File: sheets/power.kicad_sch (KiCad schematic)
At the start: 73 parts, among them SW2 FCC-0001SW, T1 COIL, U11 74LS05, U12 74LS06, U28 PC4741, U29 PC4741, U33 74AS04, U37 LM2576T-5, U38 74HC32, U8 74HC04, U80 74HC04

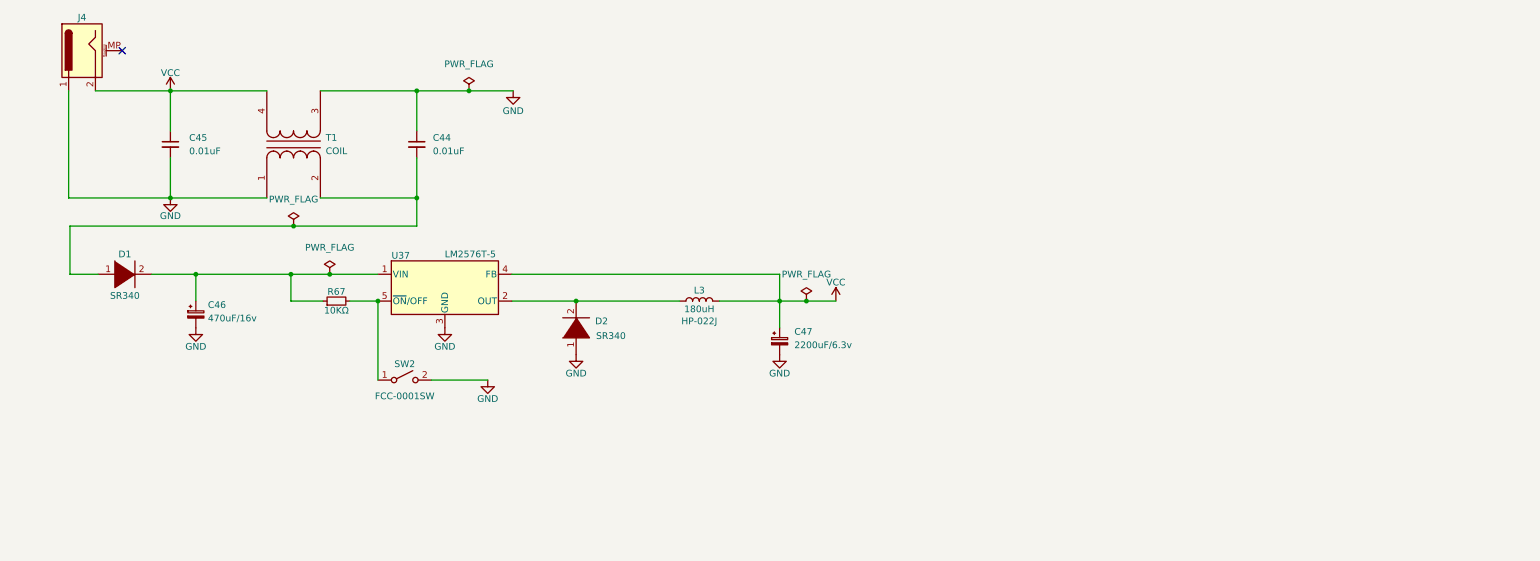
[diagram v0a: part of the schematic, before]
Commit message: Power Circuit Update 1
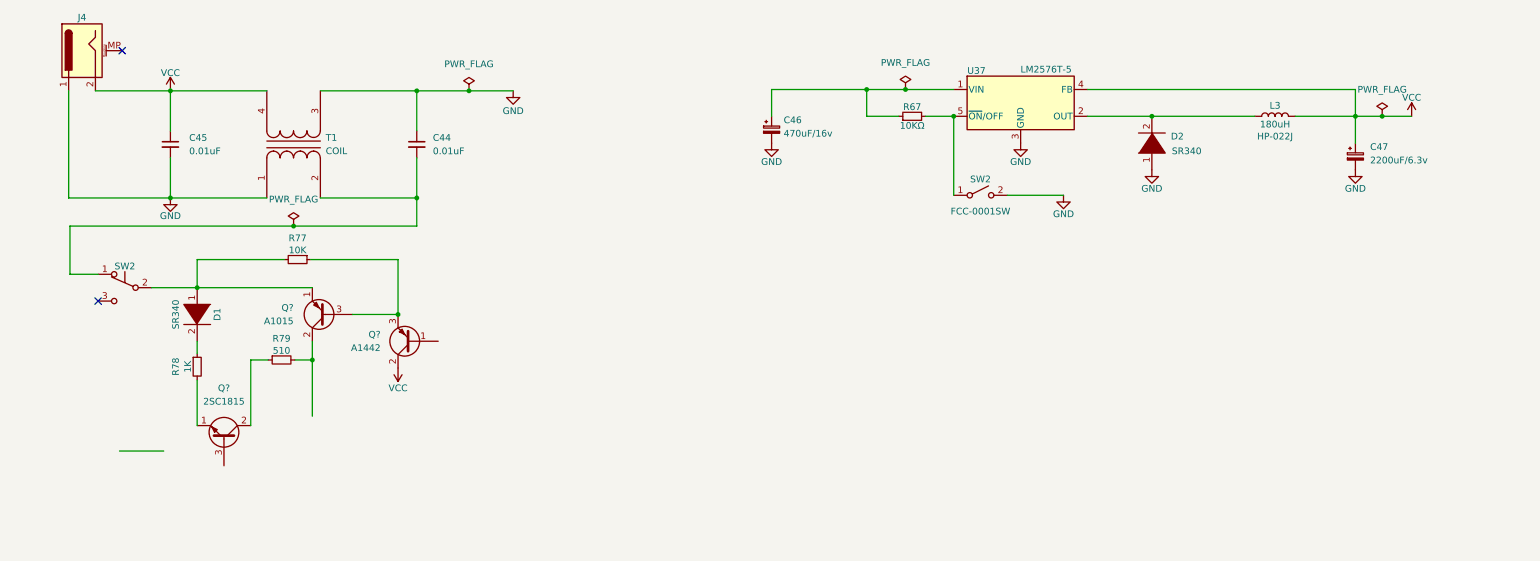
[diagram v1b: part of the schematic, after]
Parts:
- added Q?: A1442, symbol Device:Q_PNP_BCE
- added Q?: A1015, Package_TO_SOT_THT:TO-92_Inline, symbol Transistor_BJT:2SA1015
- added Q?: 2SC1815, Package_TO_SOT_THT:TO-92_Inline, symbol Transistor_BJT:2SC1815
- added R77: 10K, symbol Device:R_Small
- added R78: 1K, symbol Device:R_Small
- added R79: 510, symbol Device:R_Small
- added SW2: ~, symbol Switch:SW_Push_SPDT
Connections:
- net VCC: now also Q?.2 (C)
- net at C46.1, R67.1, U37.1 (VIN): no longer D1.2 (A)
- net at C44.2, T1.2 (AB): now also SW2.1 (A); no longer D1.1 (K)
- new net: Q?.3 (B), Q?.3 (E), R77.1
- new net: D1.1 (K), Q?.1 (E), R77.2, SW2.2 (B)
- new net: Q?.2 (C), R79.2
- new net: Q?.1 (E), R78.2
- new net: Q?.2 (C), R79.1
- new net: D1.2 (A), R78.1
- no-connect marks 10 -> 11
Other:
- moved on the sheet: C46, C47, D1, D2, L3, R67, SW2, U37
